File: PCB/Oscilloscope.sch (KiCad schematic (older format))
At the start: 27 parts

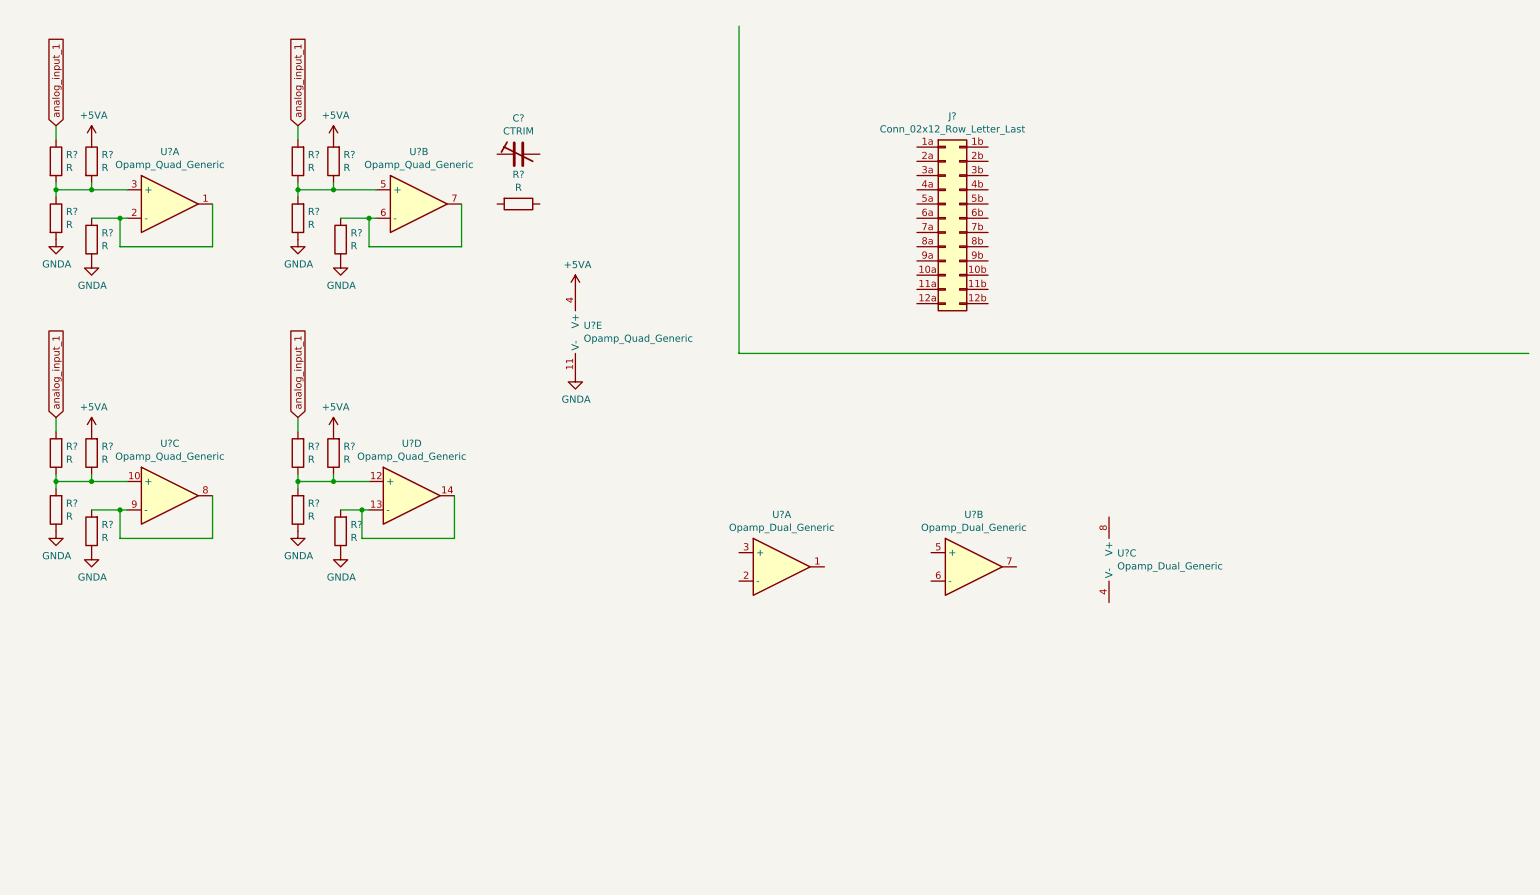
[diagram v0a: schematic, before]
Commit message: Advancing in the schmatic. Power to be finished
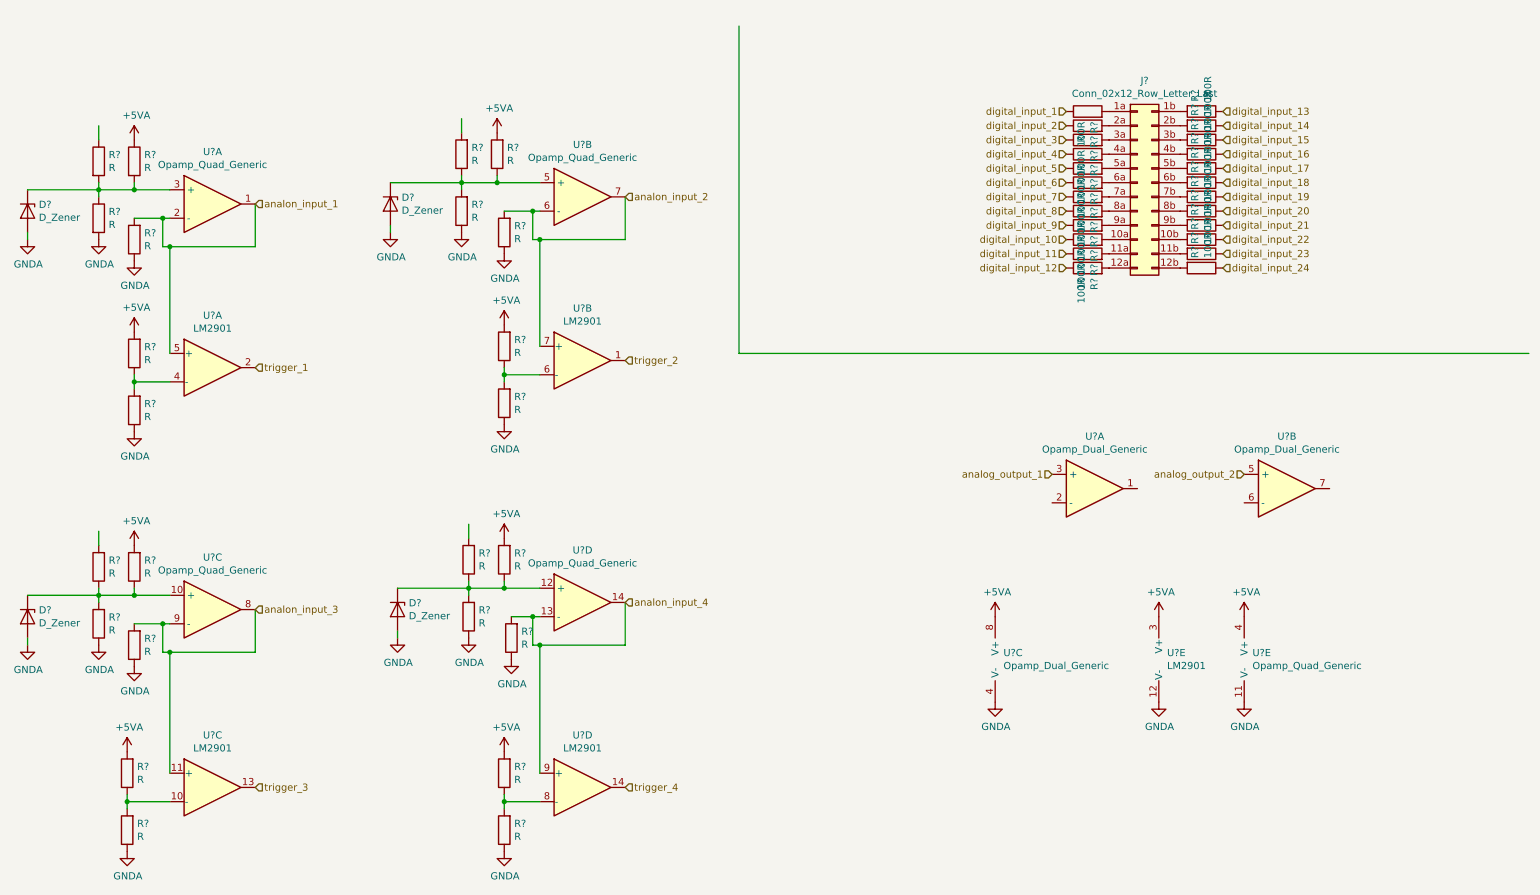
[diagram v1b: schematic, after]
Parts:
- removed C?: CTRIM, symbol Device:CTRIM
- removed R?: R, symbol Device:R
- added D? (x4): D_Zener, symbol Device:D_Zener
- added R? (x9): R, symbol Device:R
- added R? (x23): 100R, symbol Device:R
- added U? (x5): LM2901, symbol Comparator:LM2901
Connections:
- net labels added: analog_output_1, analog_output_2, analon_input_1, analon_input_2, analon_input_3, analon_input_4, digital_input_1, digital_input_10, digital_input_11, digital_input_12, digital_input_13, digital_input_14, digital_input_15, digital_input_16, digital_input_17, digital_input_18, digital_input_19, digital_input_2, digital_input_20, digital_input_21, digital_input_22, digital_input_23, digital_input_24, digital_input_3, digital_input_4, digital_input_5, digital_input_6, digital_input_7, digital_input_8, digital_input_9, trigger_1, trigger_2, trigger_3, trigger_4
- net labels removed: analog_input_1
- wire segments 46 -> 74
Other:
- moved on the sheet: J?, R?, U?A, U?B, U?C, U?D, U?E
